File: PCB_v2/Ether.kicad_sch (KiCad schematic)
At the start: 30 parts, among them J9 RJ45_Bel_SI-60062-F, U8 W5500, Y3 25M

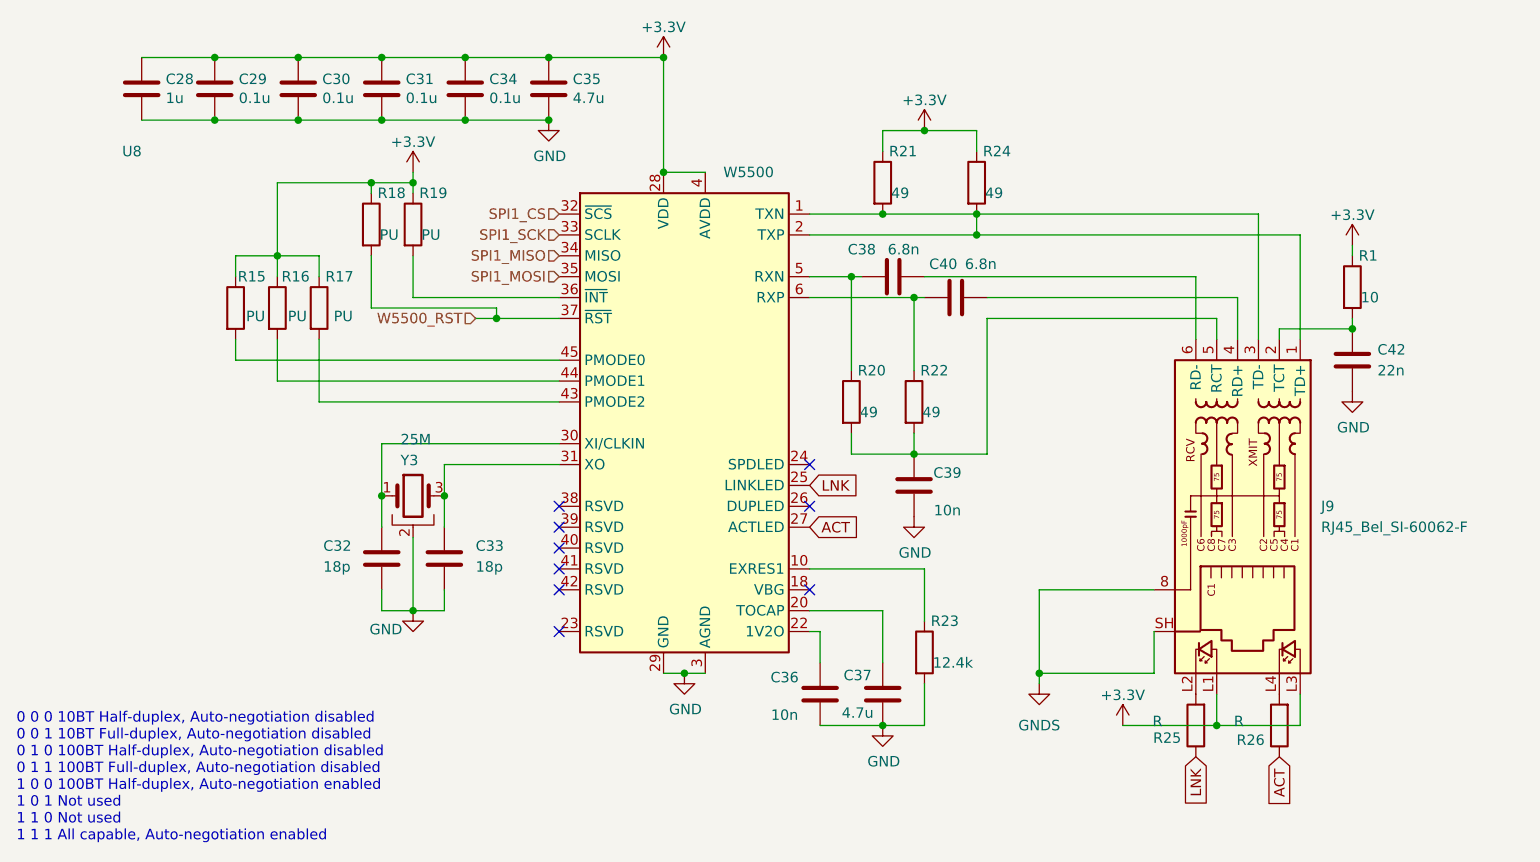
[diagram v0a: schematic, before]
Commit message: 動いたからコミット
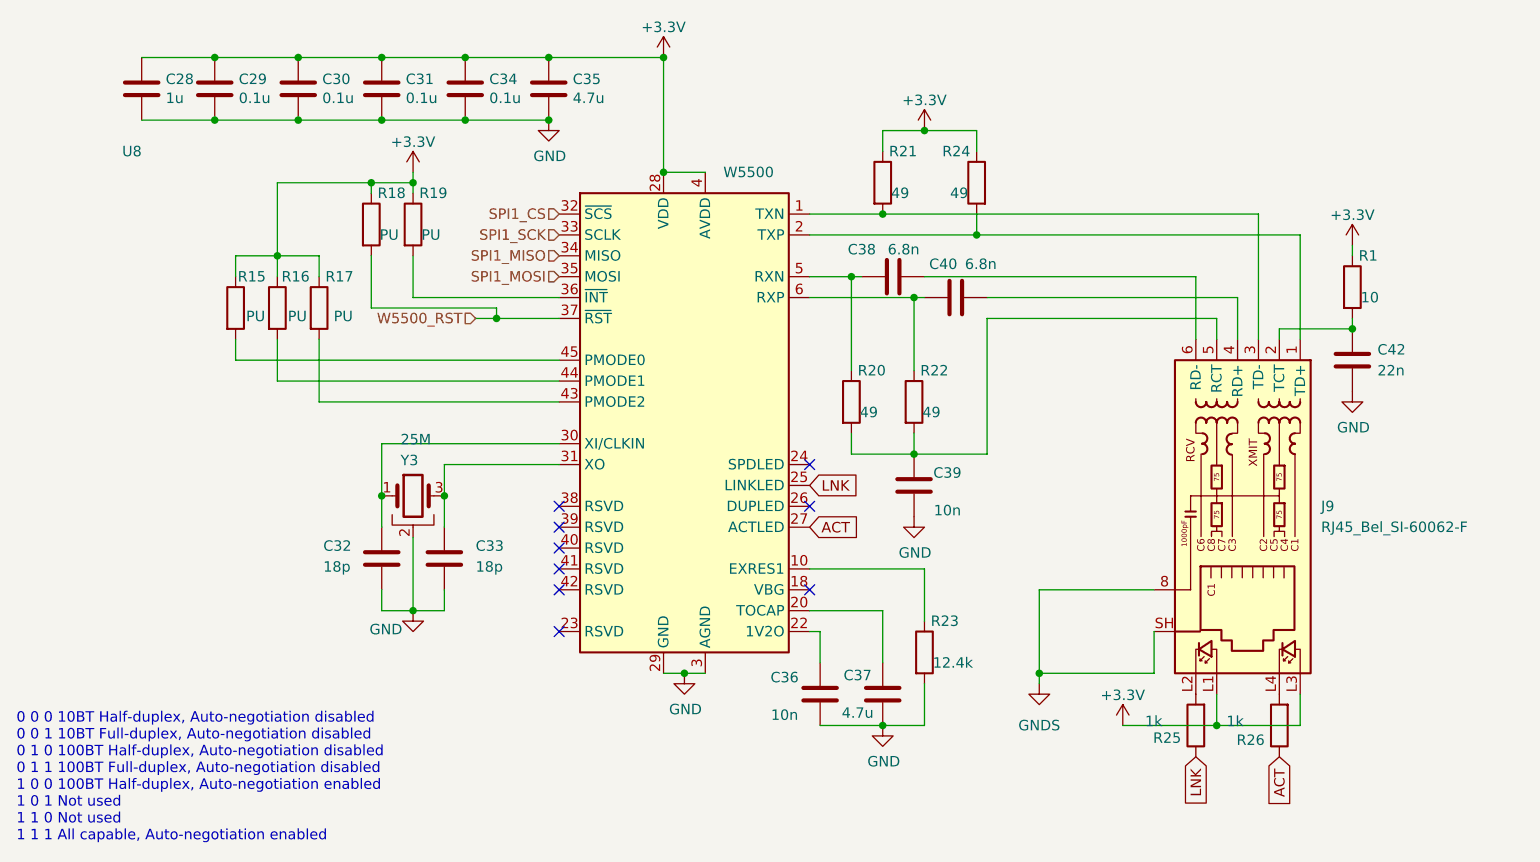
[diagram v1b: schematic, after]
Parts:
- R25, R26: value R -> 1k
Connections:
- net at J9.1 (TD+), R24.2, U8.2 (TXP): no longer J9.3 (TD-), R21.2, U8.1 (TXN)
- new net: J9.3 (TD-), R21.2, U8.1 (TXN)
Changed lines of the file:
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@@
-	)
-	(junction
-		(at 172.72 73.66)
-		(diameter 0)
-		(color 0 0 0 0)
 	)
 	(junction
@@
 	(wire
 		(pts
-			(xy 172.72 73.66) (xy 207.01 73.66)
-		)
-		(stroke
-			(width 0)
-			(type default)
-		)
-	)
-	(wire
-		(pts
 			(xy 152.4 124.46) (xy 153.67 124.46)
 		)
@@
 	(wire
 		(pts
-			(xy 161.29 73.66) (xy 172.72 73.66)
+			(xy 161.29 73.66) (xy 207.01 73.66)
 		)
 		(stroke
@@
 		(lib_id "Device:R")
 		(at 172.72 69.85 0)
+		(mirror y)
 		(unit 1)
 		(exclude_from_sim no)
@@
 		(dnp no)
 		(property "Reference" "R24"
-			(at 173.482 66.04 0)
+			(at 171.958 66.04 0)
 			(effects
 				(font
@@
 		)
 		(property "Value" "49"
-			(at 173.736 71.12 0)
+			(at 171.704 71.12 0)
 			(effects
 				(font
@@
 		)
 		(property "Footprint" "Resistor_SMD:R_0402_1005Metric"
-			(at 170.942 69.85 90)
+			(at 174.498 69.85 90)
 			(effects
 				(font
@@
 			)
 		)
-		(property "Value" "R"
+		(property "Value" "1k"
 			(at 205.232 135.382 0)
 			(effects
@@
 			)
 		)
-		(property "Value" "R"
+		(property "Value" "1k"
 			(at 195.326 135.382 0)
 			(effects
